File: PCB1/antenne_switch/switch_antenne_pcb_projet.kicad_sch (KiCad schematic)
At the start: 10 parts, among them J1 Conn_Coaxial, J2 Conn_Coaxial

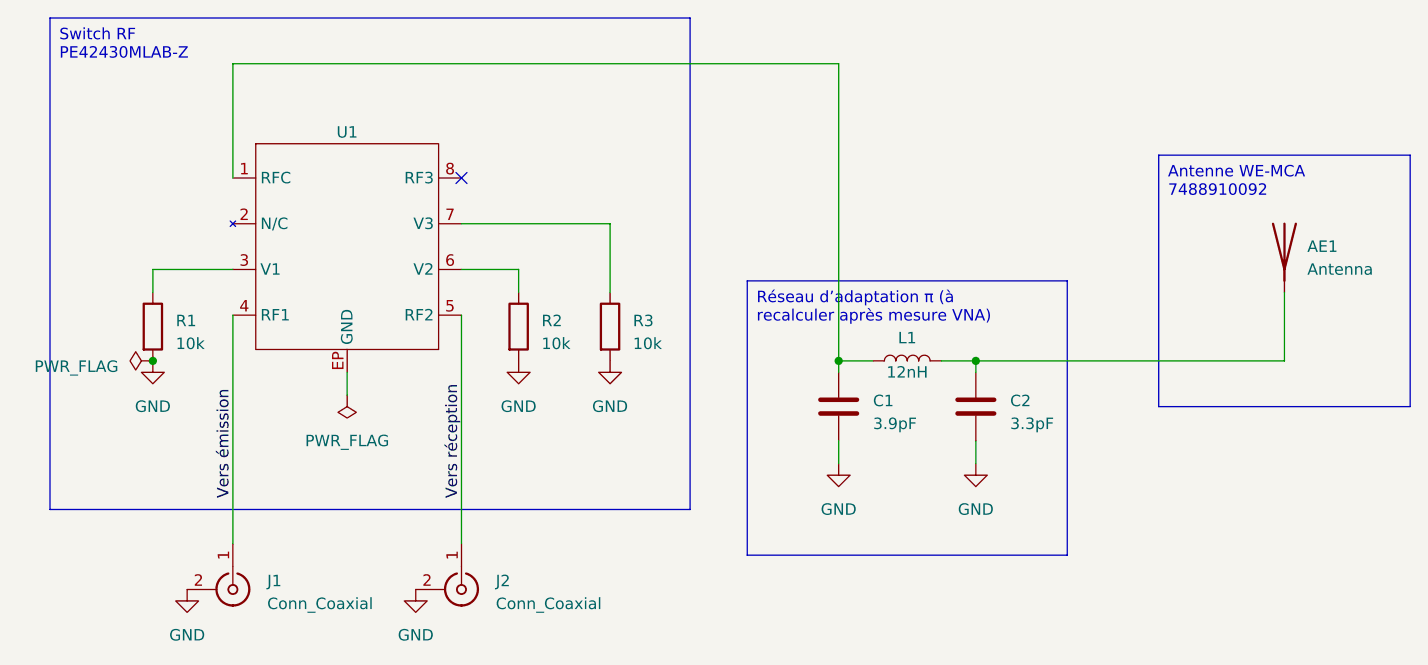
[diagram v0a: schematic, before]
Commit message: pcb2
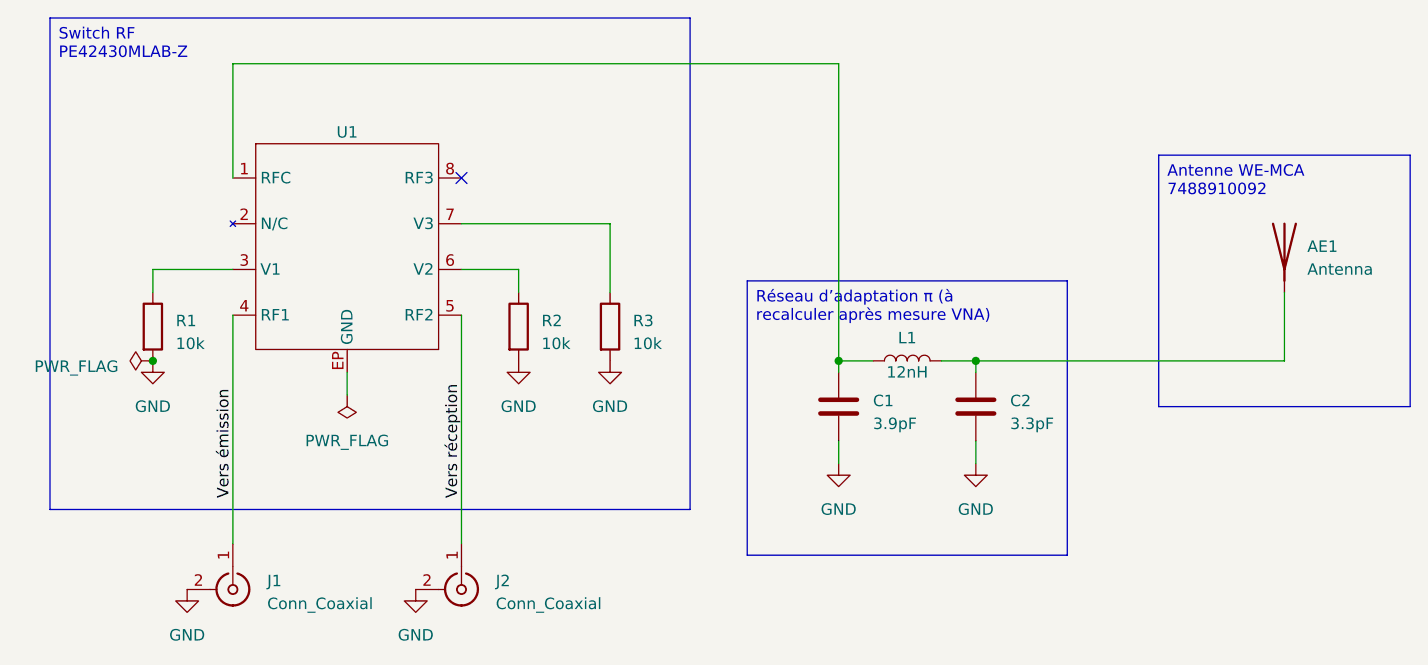
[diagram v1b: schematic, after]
